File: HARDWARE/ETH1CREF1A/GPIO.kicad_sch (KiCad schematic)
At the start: 7 parts, among them U501 74HCT595PW, U503 SN74LVC1T45DRLR, U504 SN74LVC1T45DRLR, U505 SN74LVC1T45DRLR, U506 SN74LVC1T45DRLR

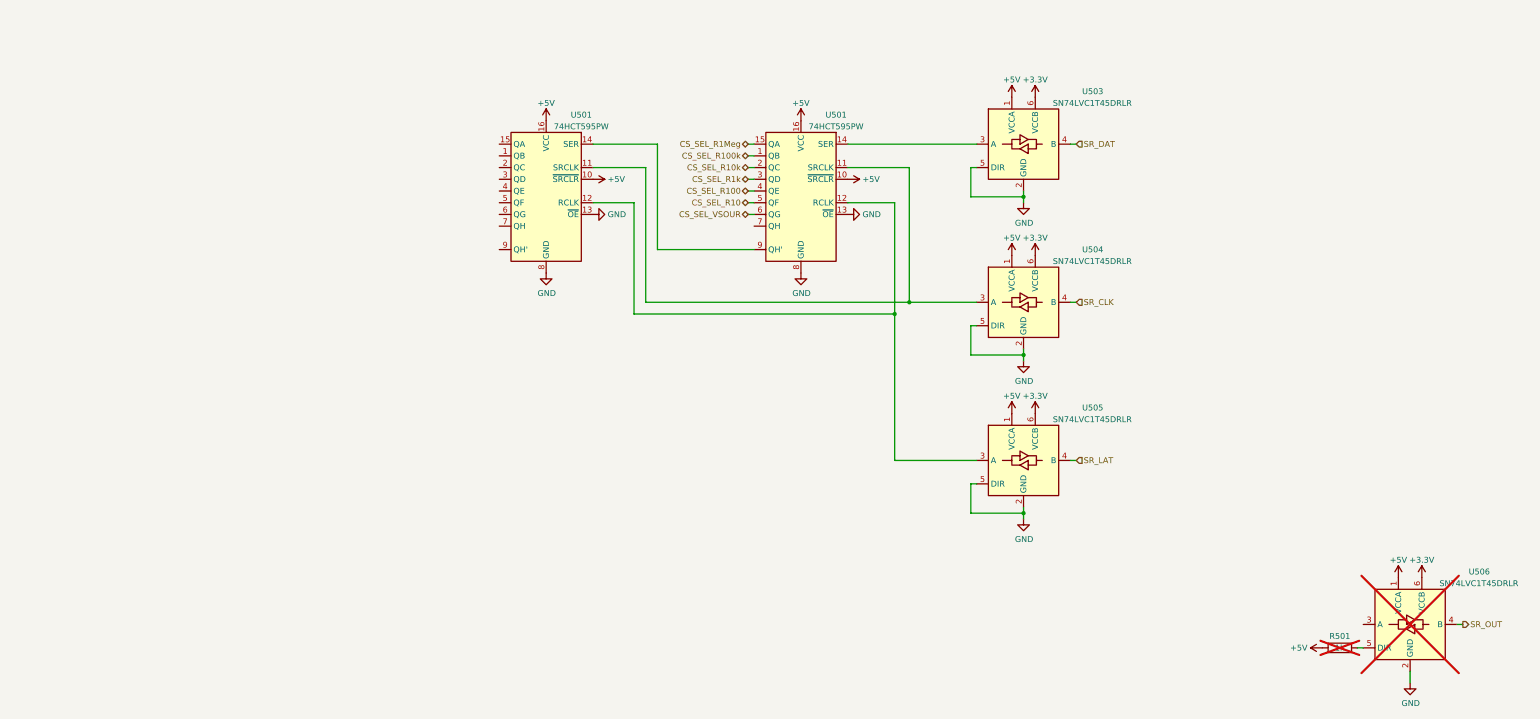
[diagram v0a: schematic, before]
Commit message: Hardware
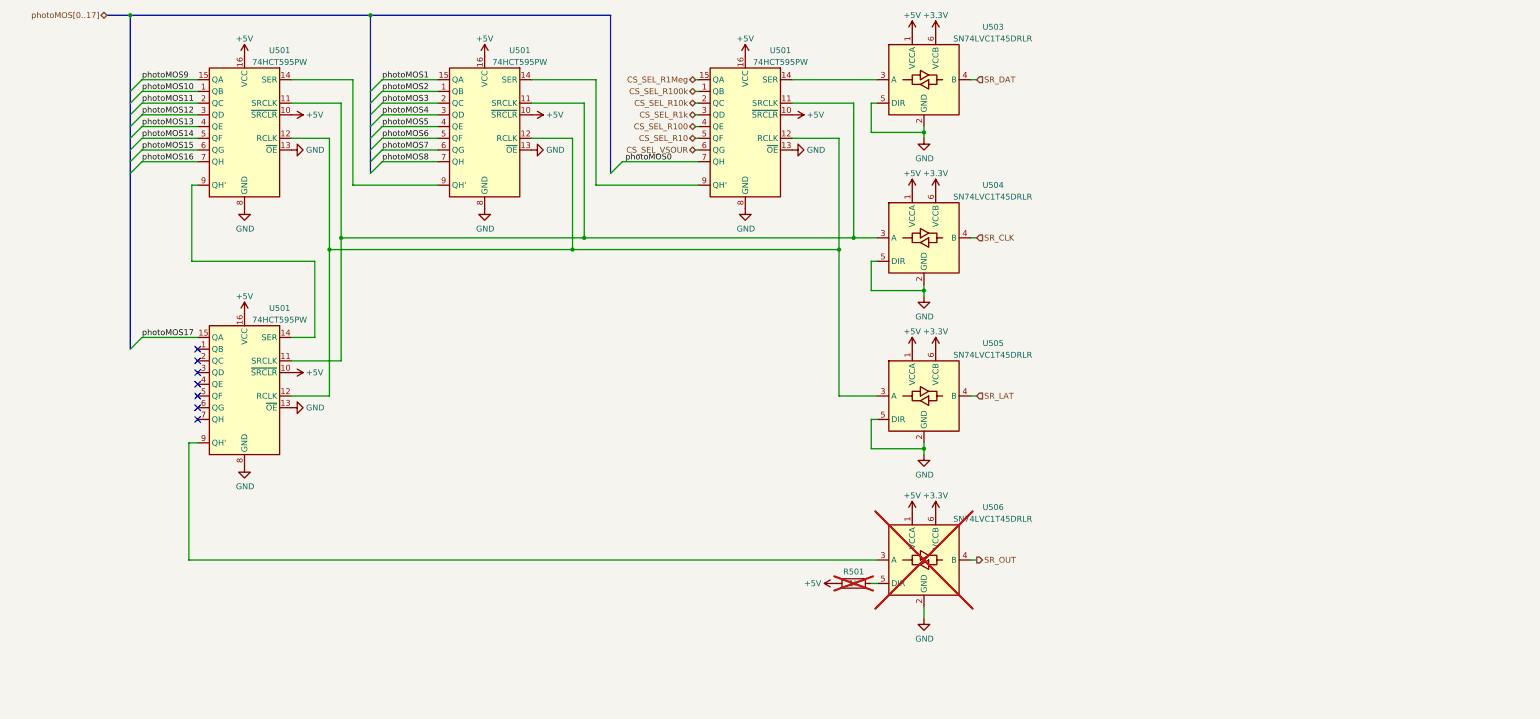
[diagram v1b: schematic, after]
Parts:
- added U501 (x2): 74HCT595PW, Package_SO:TSSOP-16_4.4x5mm_P0.65mm, symbol 74xx:74HCT595
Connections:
- net +5V: now also U501.10 (~{SRCLR}), U501.10 (~{SRCLR}), U501.16 (VCC), U501.16 (VCC)
- net GND: now also U501.13 (~{OE}), U501.13 (~{OE}), U501.8 (GND), U501.8 (GND)
- net at U501.11 (SRCLK), U501.11 (SRCLK), U504.3 (A): now also U501.11 (SRCLK), U501.11 (SRCLK)
- net at U501.12 (RCLK), U501.12 (RCLK), U505.3 (A): now also U501.12 (RCLK), U501.12 (RCLK)
- net photoMOS0: now reaches U501.7 (QH)
- net at U506.3 (A): now also U501.9 (QH')
- net photoMOS2: now reaches U501.1 (QB)
- net photoMOS1: now reaches U501.15 (QA)
- net photoMOS3: now reaches U501.2 (QC)
- net photoMOS4: now reaches U501.3 (QD)
- net photoMOS5: now reaches U501.4 (QE)
- net photoMOS6: now reaches U501.5 (QF)
- net photoMOS7: now reaches U501.6 (QG)
- net photoMOS8: now reaches U501.7 (QH)
- net at U501.9 (QH'): now also U501.14 (SER)
- new net: U501.14 (SER), U501.9 (QH')
- new net photoMOS10: U501.1 (QB)
- new net photoMOS11: U501.2 (QC)
- new net photoMOS12: U501.3 (QD)
- new net photoMOS13: U501.4 (QE)
- new net photoMOS14: U501.5 (QF)
- new net photoMOS15: U501.6 (QG)
- new net photoMOS16: U501.7 (QH)
- new net photoMOS17: U501.15 (QA)
- new net photoMOS9: U501.15 (QA)
- no-connect marks 0 -> 7
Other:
- moved on the sheet: R501, U501, U503, U504, U505, U506
